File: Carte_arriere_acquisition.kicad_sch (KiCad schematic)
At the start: 18 parts, among them J1 Screw_Terminal_01x02, J2 Vers_BMS, J3 Vers_Thermistor, J4 Vers_Capteur_Hall, J5 Conn_01x04_Pin, J6 Conn_01x04_Pin, U1 ESP32-DEVKITC-32E, U2 SN65HVD230, U3 MAX3485, U4 module_mpu6050

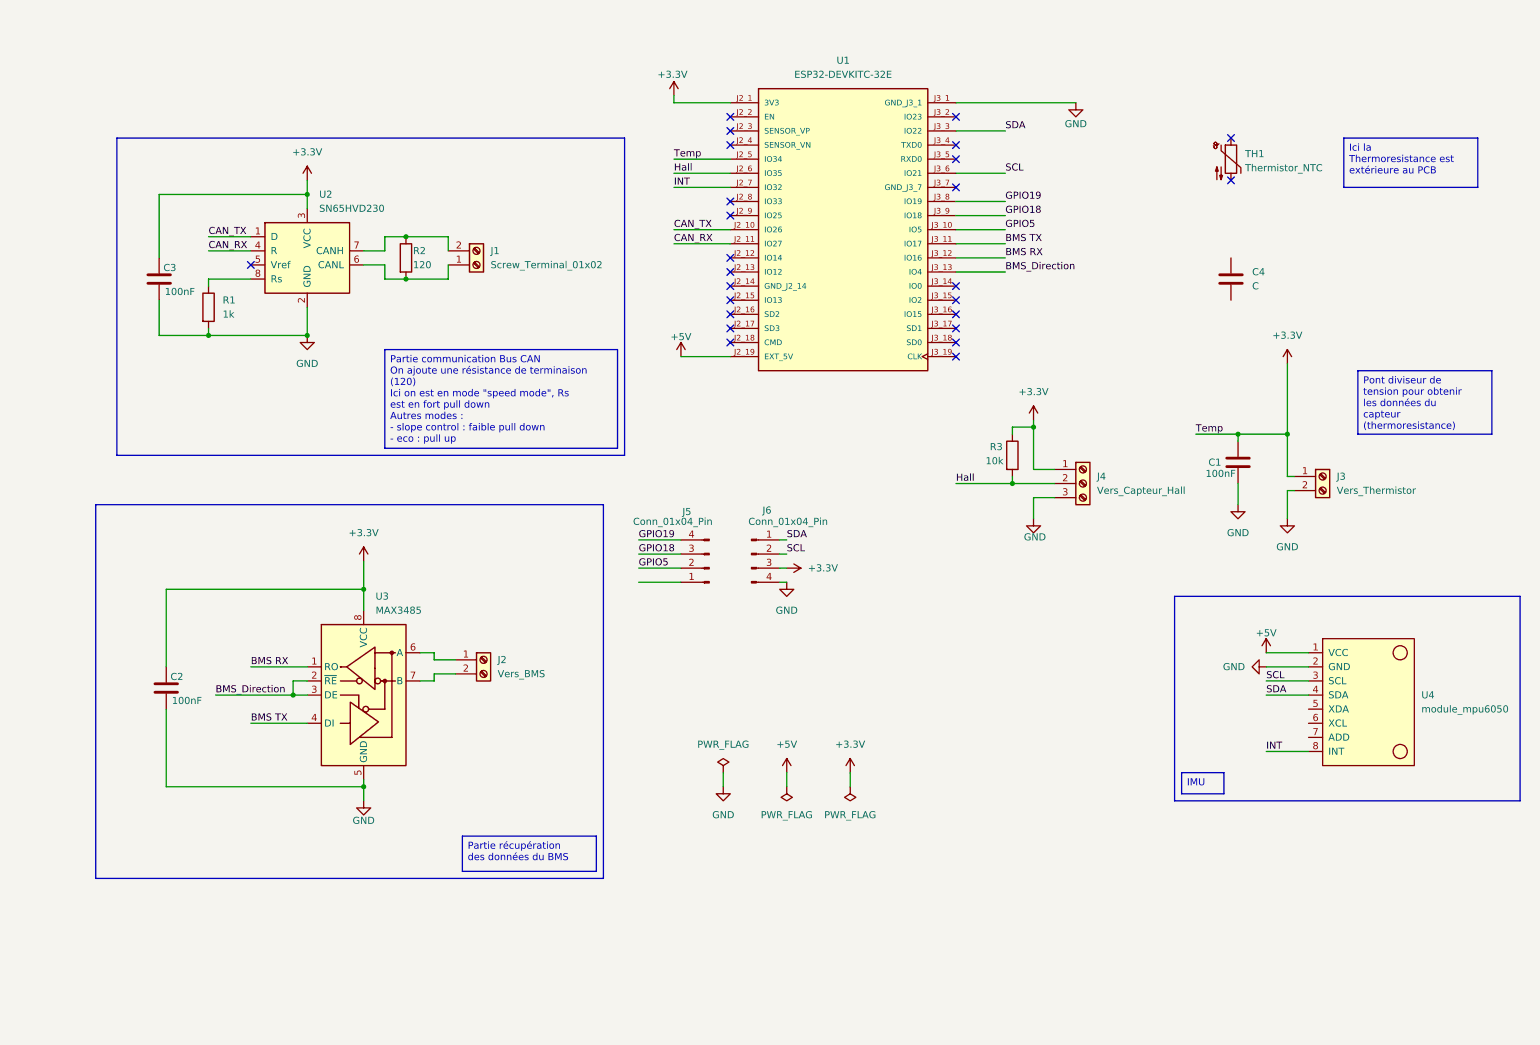
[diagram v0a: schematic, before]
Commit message: Modif PCB
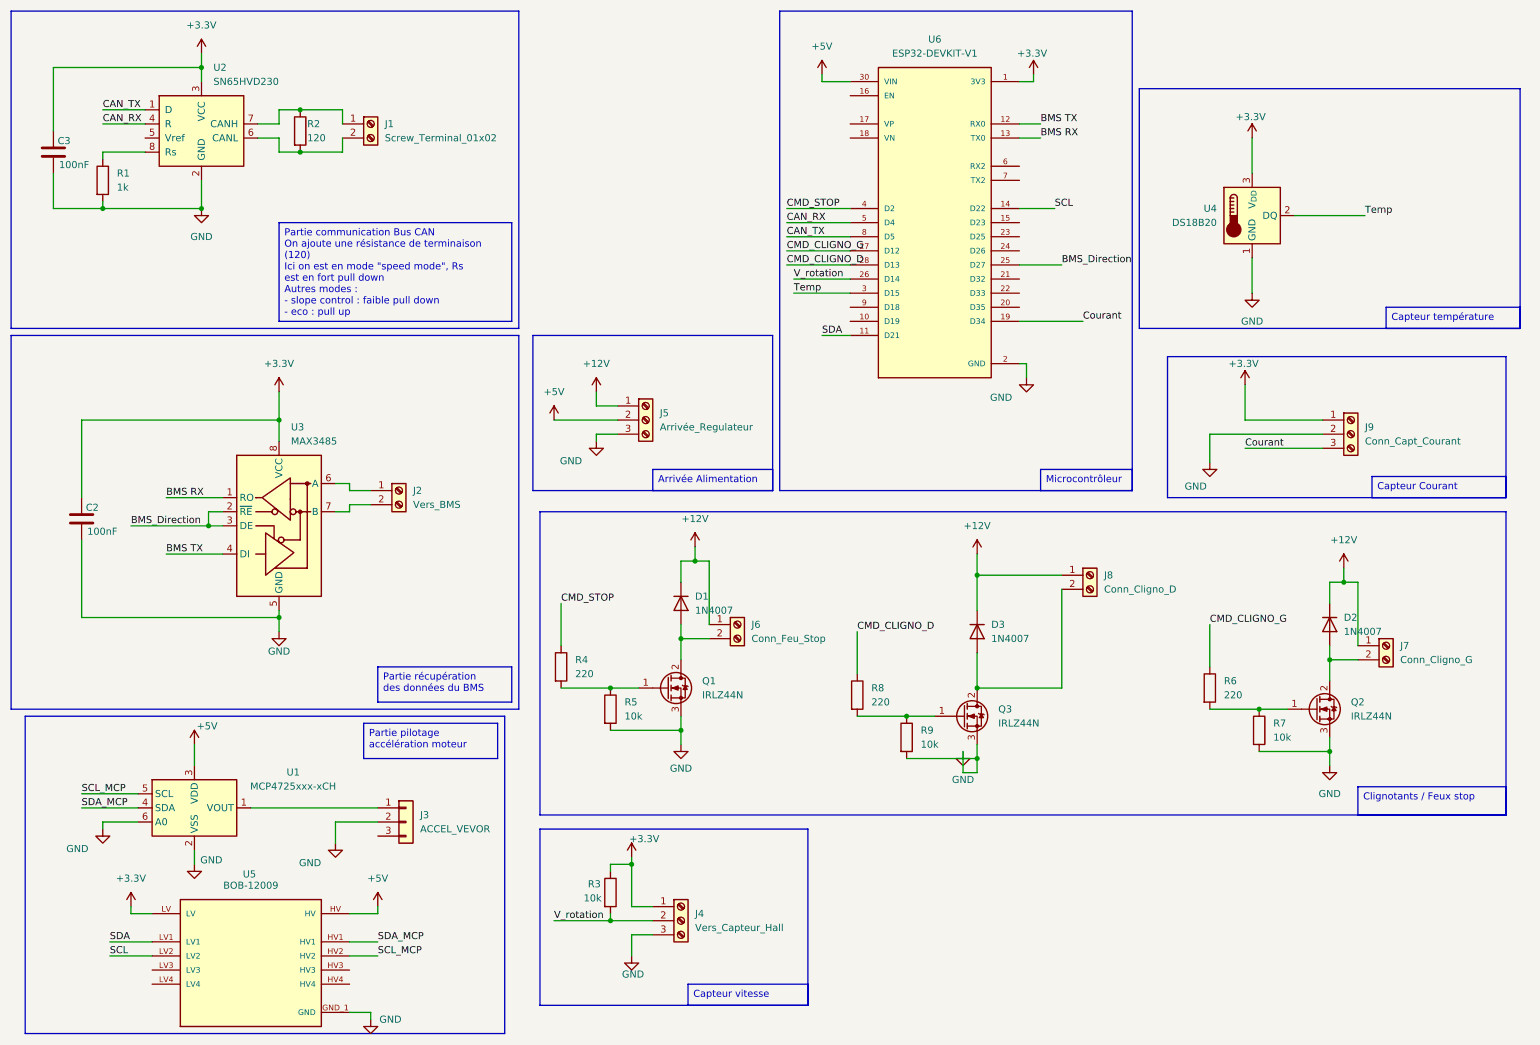
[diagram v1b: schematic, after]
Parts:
- removed C1: 100nF, Capacitor_SMD:C_0805_2012Metric_Pad1.18x1.45mm_HandSolder, symbol Device:C
- removed C4: C, symbol Device:C
- removed J3: Vers_Thermistor, TerminalBlock_Phoenix:TerminalBlock_Phoenix_MKDS-1,5-2_1x02_P5.00mm_Horizontal, symbol Connector:Screw_Terminal_01x02
- removed J5, J6: Conn_01x04_Pin, Connector_PinHeader_1.27mm:PinHeader_1x04_P1.27mm_Vertical, symbol Connector:Conn_01x04_Pin
- removed TH1: Thermistor_NTC, symbol Device:Thermistor_NTC
- removed U1: ESP32-DEVKITC-32E, ESP32-DEVKITC-32E:MODULE_ESP32-DEVKITC-32E, symbol ESP32-DEVKITC-32E:ESP32-DEVKITC-32E
- removed U4: module_mpu6050, usini_sensors:module_mpu6050, symbol usini_sensors:module_mpu6050
- added D1, D2, D3: 1N4007, Diode_THT:D_DO-41_SOD81_P10.16mm_Horizontal, symbol Diode:1N4007
- added J3: ACCEL_VEVOR, symbol Connector_Generic:Conn_01x03
- added J5: Arrivée_Regulateur, symbol Connector:Screw_Terminal_01x03
- added J6: Conn_Feu_Stop, symbol Connector:Screw_Terminal_01x02
- added J7: Conn_Cligno_G, symbol Connector:Screw_Terminal_01x02
- added J8: Conn_Cligno_D, symbol Connector:Screw_Terminal_01x02
- added J9: Conn_Capt_Courant, symbol Connector:Screw_Terminal_01x03
- added Q1, Q2, Q3: IRLZ44N, Package_TO_SOT_THT:TO-220-3_Vertical, symbol Transistor_FET:IRLZ44N
- added R4, R6, R8: 220, symbol Device:R
- added R5, R7, R9: 10k, symbol Device:R
- added U1: MCP4725xxx-xCH, Package_TO_SOT_SMD:SOT-23-6, symbol Analog_DAC:MCP4725xxx-xCH
- added U4: DS18B20, Package_TO_SOT_THT:TO-92_Inline, symbol Sensor_Temperature:DS18B20
- added U5: BOB-12009, BOB-12009:CONV_BOB-12009, symbol BOB-12009:BOB-12009
- added U6: ESP32-DEVKIT-V1, ESP32-DEVKIT-V1:MODULE_ESP32_DEVKIT_V1, symbol ESP32-DEVKIT-V1:ESP32-DEVKIT-V1
- C2, C3: footprint Capacitor_SMD:C_0805_2012Metric_Pad1.18x1.45mm_HandSolder -> (none)
- J1, J2: footprint TerminalBlock_Phoenix:TerminalBlock_Phoenix_MKDS-1,5-2_1x02_P5.00mm_Horizontal -> (none)
- J4: footprint TerminalBlock_Phoenix:TerminalBlock_Phoenix_MKDS-1,5-3_1x03_P5.00mm_Horizontal -> (none)
- R1, R2, R3: footprint Resistor_SMD:R_0805_2012Metric_Pad1.20x1.40mm_HandSolder -> (none)
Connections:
- net +3.3V: now also J9.1 (Pin_1), U4.3 (V_{DD}), U5.LV, U6.1 (3V3)
- net +5V: now also J5.2 (Pin_2), U1.3 (VDD), U5.HV, U6.30 (VIN)
- net BMS RX: now also U6.13 (TX0)
- net BMS TX: now also U6.12 (RX0)
- net BMS_Direction: now also U6.25 (D27)
- net CAN_RX: now also U6.5 (D4)
- net CAN_TX: now also U6.8 (D5)
- net GND: now also J3.2 (Pin_2), J5.3 (Pin_3), J9.2 (Pin_2), Q1.3 (S), Q2.3 (S), Q3.3 (S), R5.2, R7.2, R9.2, U1.2 (VSS), U1.6 (A0), U4.1 (GND), U5.GND_1 (GND), U5.GND_2 (GND), U6.2 (GND), U6.29 (GND)
- net SCL: now also U5.LV2, U6.14 (D22)
- net SDA: now also U5.LV1, U6.11 (D21)
- net at R2.1, U2.7 (CANH): now also J1.1 (Pin_1); no longer J1.2 (Pin_2)
- net at R2.2, U2.6 (CANL): now also J1.2 (Pin_2); no longer J1.1 (Pin_1)
- net Hall renamed V_rotation
- net V_rotation: now also U6.26 (D14)
- new net: D1.2 (A), J6.2 (Pin_2), Q1.2 (D)
- new net: D3.2 (A), J8.2 (Pin_2), Q3.2 (D)
- new net: Q1.1 (G), R4.2, R5.1
- new net: D2.2 (A), J7.2 (Pin_2), Q2.2 (D)
- new net: J3.1 (Pin_1), U1.1 (VOUT)
- new net: Q3.1 (G), R8.2, R9.1
- new net: Q2.1 (G), R6.2, R7.1
- new net +12V: D1.1 (K), D2.1 (K), D3.1 (K), J5.1 (Pin_1), J6.1 (Pin_1), J7.1 (Pin_1), J8.1 (Pin_1)
- new net CMD_CLIGNO_D: R8.1, U6.28 (D13)
- new net CMD_CLIGNO_G: R6.1, U6.27 (D12)
- new net CMD_STOP: R4.1, U6.4 (D2)
- new net Courant: J9.3 (Pin_3), U6.19 (D34)
- new net SCL_MCP: U1.5 (SCL), U5.HV2
- new net SDA_MCP: U1.4 (SDA), U5.HV1
- new net Temp: U4.2 (DQ), U6.3 (D15)
- no-connect marks 25 -> 0
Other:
- moved on the sheet: C2, C3, J1, J2, J4, R1, R2, R3, U2, U3
